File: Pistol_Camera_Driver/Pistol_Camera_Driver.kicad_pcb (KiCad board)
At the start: 2 copper layers, 86.6 x 46.1 mm, 104 parts, among them J1 Screw_Terminal_01x02, J11 Screw_Terminal_01x02, J12 Screw_Terminal_01x02, J13 I2C, J14 Screw_Terminal_01x02, J15 Screw_Terminal_01x02, J16 Screw_Terminal_01x02, J17 Screw_Terminal_01x02, J18 Screw_Terminal_01x02, J19 I2C, J2 Objective, J3 Screw_Terminal_01x02, J4 Screw_Terminal_01x02, J5 Screw_Terminal_01x02, J6 Joystick, J7 Screw_Terminal_01x02, J8 Screw_Terminal_01x02, J9 Screw_Terminal_01x02, U12 MT3608, U2 XL1509-5.0, U4 DRV8834PWP, U5 DRV8834PWP

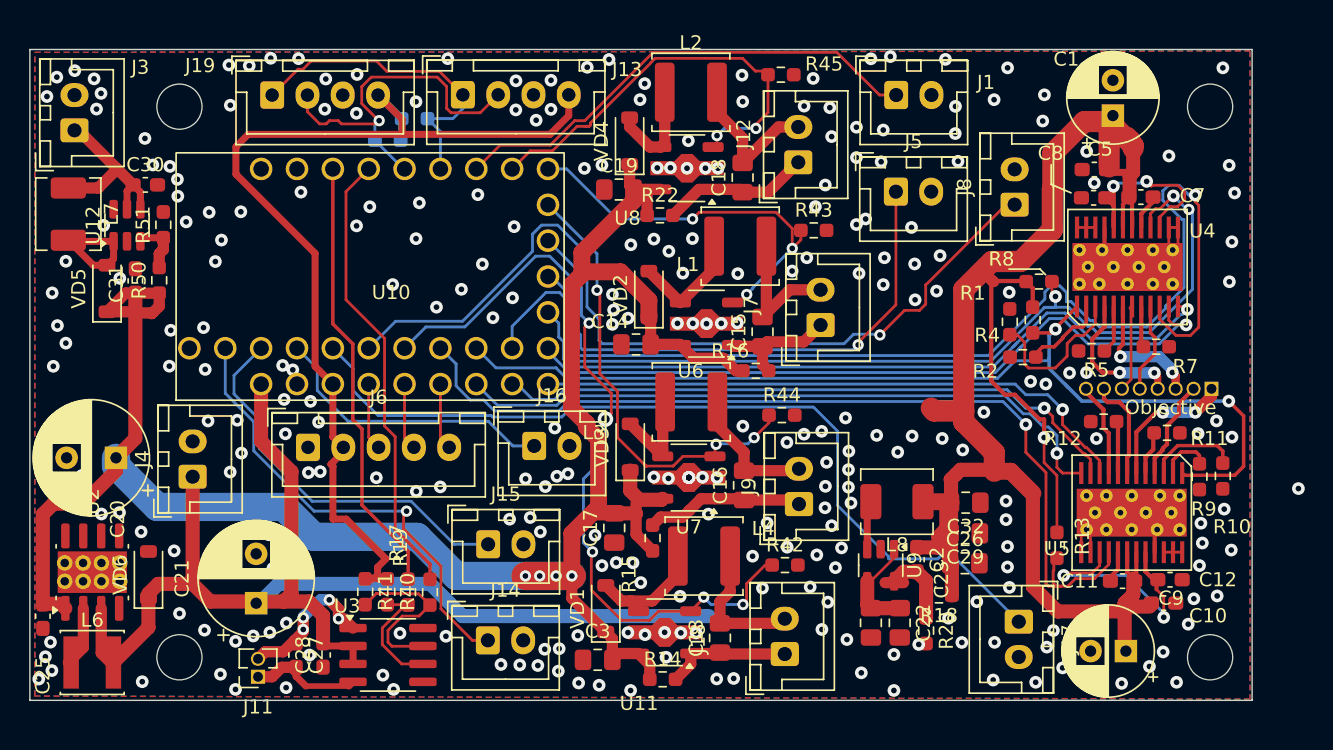
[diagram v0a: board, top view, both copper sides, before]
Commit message: v0.9 actual state
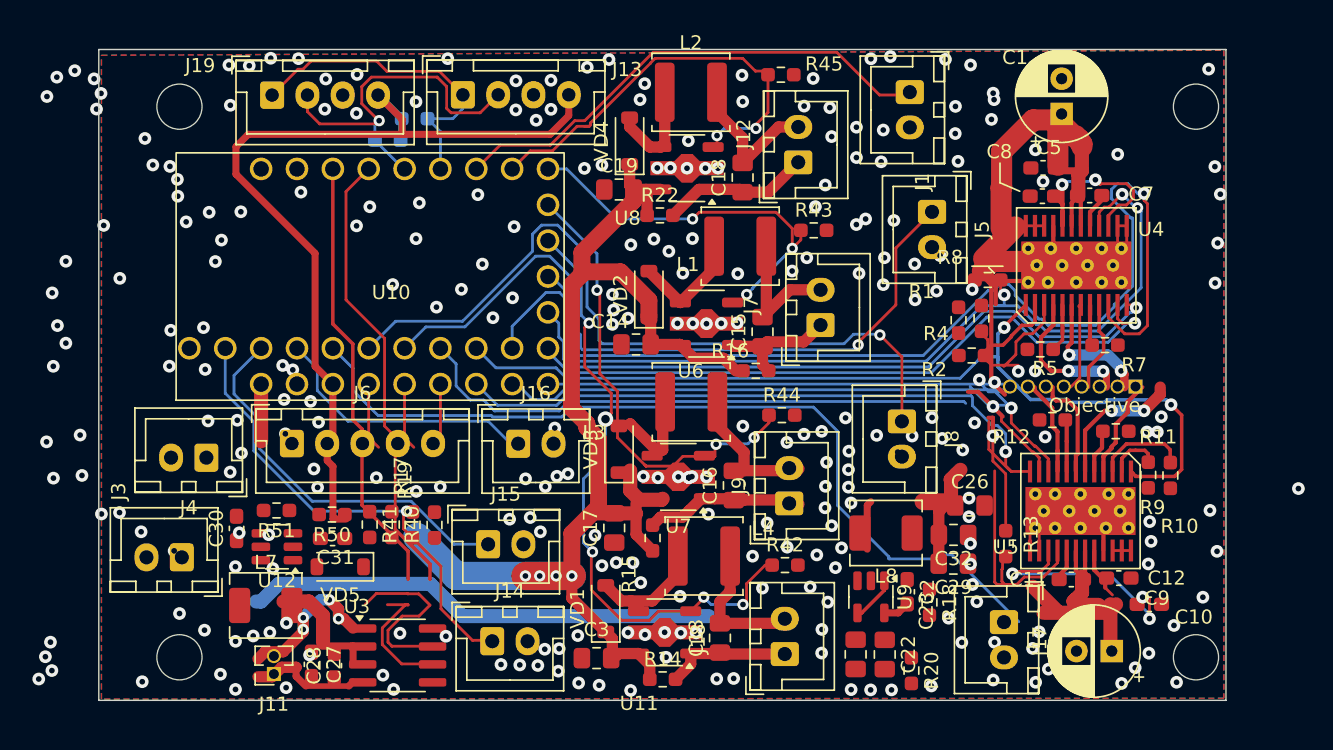
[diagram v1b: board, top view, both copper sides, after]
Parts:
- removed C20: 470uF, Capacitor_THT:CP_Radial_D8.0mm_P3.50mm
- removed C21: 330uF, Capacitor_THT:CP_Radial_D8.0mm_P3.50mm
- removed C25: 0.1, Capacitor_SMD:C_0603_1608Metric_Pad1.08x0.95mm_HandSolder
- removed L6: 22u, Inductor_SMD:L_Sunlord_SWPA4012S
- removed U2: XL1509-5.0, Package_SO:SOIC-8-1EP_3.9x4.9mm_P1.27mm_EP2.95x4.9mm_Mask2.71x3.4mm_ThermalVias
- removed VD6: CDBA3100-HF, Diode_SMD:D_SOD-123
- moved J3 31.2 mm to (40.8, 67.6), turned to 180 degrees
- moved L7 31.0 mm to (46.8, 71.0), turned to 0 degrees
- moved VD5 25.7 mm to (52.0, 68.2), turned to 180 degrees
- moved C30 25.2 mm to (44.7, 65.5), turned to 90 degrees
- moved U12 25.1 mm to (47.5, 66.8), turned to 180 degrees
- moved C31 23.0 mm to (51.5, 66.2), turned to 180 degrees
- moved R51 21.8 mm to (47.5, 64.2), turned to 180 degrees
- moved R50 20.6 mm to (51.4, 64.5), turned to 180 degrees
- moved J8 17.3 mm to (91.8, 57.9), turned to -90 degrees
- moved J2 5.39 mm to (108.4, 55.5)
- moved R41 4.77 mm to (54.1, 65.2)
- moved R40 4.77 mm to (55.7, 65.2)
- moved R17 4.77 mm to (57.2, 65.3)
- moved R19 4.77 mm to (58.7, 65.3)
- moved C26 4.11 mm to (96.6, 63.9)
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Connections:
- C28 pad 2: +5V -> +3.3VP
- J4 pad 1: +5V -> VBUS
- U10 pad 32: +5V -> VBUS
- U3 pad 2: +5V -> +3.3VP
- U3 pad 3: +5V -> +3.3VP
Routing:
- net +5V: track 87.0 -> 0.00 mm
- net VPP: track 153.1 -> 92.3 mm
- net (no net): track 0.00 -> 33.5 mm
- net +3.3VP: track 132.6 -> 100.3 mm
- net VBUS: track 20.7 -> 7.26 mm
- net Net-(U12-SW): track 8.60 -> 0.00 mm
- net +3V3: track 71.5 -> 63.9 mm
- net K2: track 61.5 -> 54.1 mm
- net MOTORS_nSLEEP: track 72.6 -> 66.9 mm
- net Net-(U5-CONFIG): track 17.6 -> 12.1 mm, vias 2 -> 1
- net GND: track 17.7 -> 23.3 mm, vias 285 -> 286
- net nFLT2: track 65.6 -> 60.7 mm
- net Net-(U9-FB): track 6.74 -> 1.88 mm
- net Net-(U2-OUT): track 4.28 -> 0.00 mm
- net nEN1: track 78.9 -> 74.9 mm
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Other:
- board size 86.6 x 46.1 mm -> 79.8 x 46.1 mm
